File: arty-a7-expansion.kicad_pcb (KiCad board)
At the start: 4 copper layers, 109.4 x 40 mm, 62 parts, among them IC1 TPD8S009DSMR, J2 1140084168, J4 685119134923, J5 UE27AC54100, U1 TPS61232DRCT, U2 MAX3421EEHJ, Y1 ABM8G-12.000MHZ-18-D2Y-T

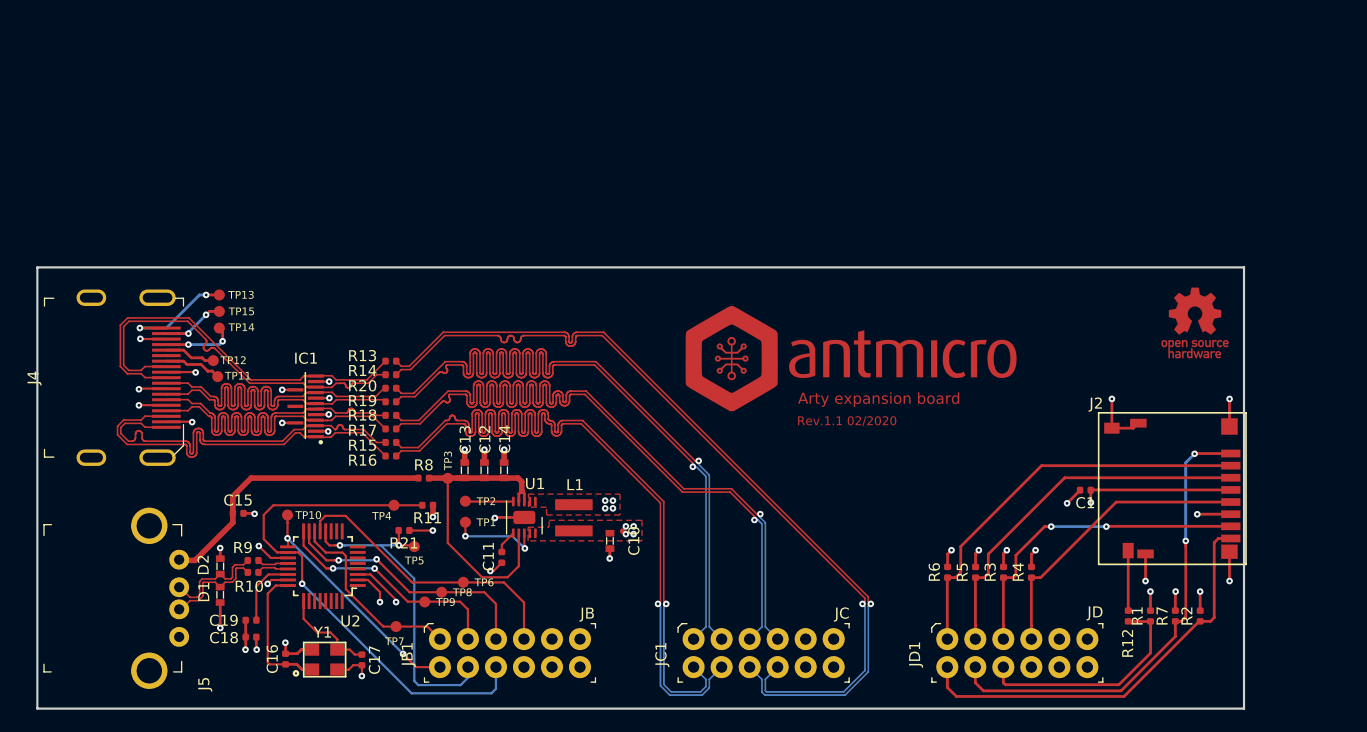
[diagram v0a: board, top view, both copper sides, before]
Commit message: Add revision 2.0.1
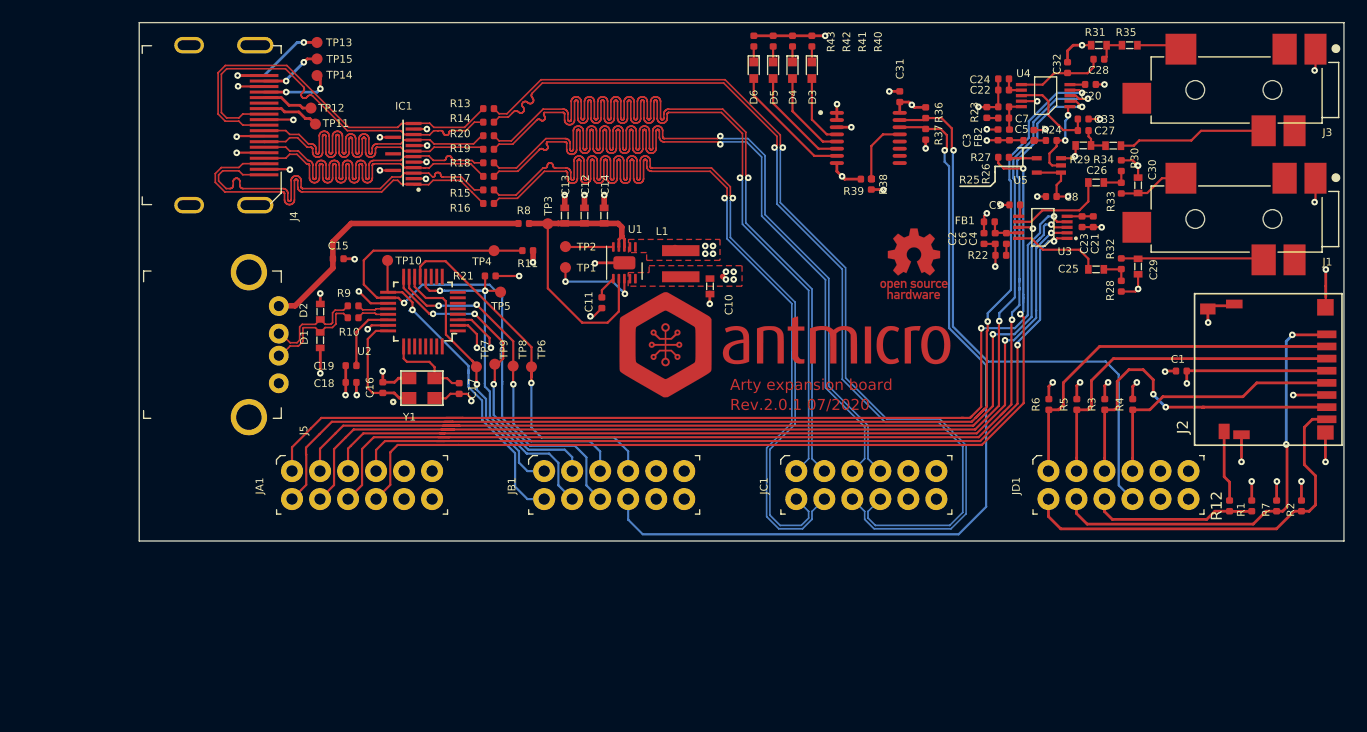
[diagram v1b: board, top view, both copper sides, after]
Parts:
- added C2: C_100n_0402_16V, arty-a7-expansion-footprints:0402-cap, F.Cu at (177.0, 81.9)
- added C20: C_10u_0402, arty-a7-expansion-footprints:0402-cap, F.Cu at (186.6, 67.9)
- added C21: C_100n_0402_16V, arty-a7-expansion-footprints:0402-cap, F.Cu at (186.9, 80.3)
- added C22: C_100n_0402_16V, arty-a7-expansion-footprints:0402-cap, F.Cu at (178.8, 68.4)
- added C23: C_10u_0402, arty-a7-expansion-footprints:0402-cap, F.Cu at (185.9, 80.3)
- added C24: C_1u_0402, arty-a7-expansion-footprints:0402-cap, F.Cu at (178.8, 67.4)
- added C25: C_3u3_0603, arty-a7-expansion-footprints:0603-cap, F.Cu at (187.1, 84.7)
- added C26: C_3u3_0603, arty-a7-expansion-footprints:0603-cap, F.Cu at (187.1, 76.8)
- added C27: C_1u_0402, arty-a7-expansion-footprints:0402-cap, F.Cu at (186.0, 72.1)
- added C28: C_1u_0402, arty-a7-expansion-footprints:0402-cap, F.Cu at (187.4, 65.6)
- added C29: C_2n7_0603, arty-a7-expansion-footprints:0603-cap, F.Cu at (190.9, 84.4)
- added C3: C_100n_0402_16V, arty-a7-expansion-footprints:0402-cap, F.Cu at (178.2, 72.5)
- added C30: C_2n7_0603, arty-a7-expansion-footprints:0603-cap, F.Cu at (190.9, 77.0)
- added C31: C_100n_0402_6V3, arty-a7-expansion-footprints:0402-cap, F.Cu at (169.3, 69.0)
- added C32: C_180p_0402, arty-a7-expansion-footprints:0402-cap, F.Cu at (184.6, 66.4)
- added C33: C_180p_0402, arty-a7-expansion-footprints:0402-cap, F.Cu at (186.0, 71.0)
- added C4: C_4u7_0402, arty-a7-expansion-footprints:0402-cap, F.Cu at (179.0, 81.9)
- added C5: C_4u7_0402, arty-a7-expansion-footprints:0402-cap, F.Cu at (178.8, 70.9)
- added C6: C_100n_0402_16V, arty-a7-expansion-footprints:0402-cap, F.Cu at (178.0, 81.9)
- added C7: C_100n_0402_16V, arty-a7-expansion-footprints:0402-cap, F.Cu at (178.8, 69.9)
- added C8: C_100n_0402_16V, arty-a7-expansion-footprints:0402-cap, F.Cu at (183.1, 78.1)
- added C9: C_10u_0402, arty-a7-expansion-footprints:0402-cap, F.Cu at (179.8, 78.8)
- added D3: LG_L29K-G2J1-24-Z, arty-a7-expansion-footprints:LED_0603, F.Cu at (161.4, 66.6)
- added D4: LG_L29K-G2J1-24-Z, arty-a7-expansion-footprints:LED_0603, F.Cu at (159.6, 66.6)
- added D5: LG_L29K-G2J1-24-Z, arty-a7-expansion-footprints:LED_0603, F.Cu at (157.9, 66.6)
- added D6: LG_L29K-G2J1-24-Z, arty-a7-expansion-footprints:LED_0603, F.Cu at (156.1, 66.6)
- added FB1: BLM15AG601SN1D, arty-a7-expansion-footprints:0402-res, F.Cu at (177.5, 80.3)
- added FB2: BLM15AG601SN1D, arty-a7-expansion-footprints:0402-res, F.Cu at (179.3, 72.5)
- added IC2: PCA9500PW, arty-a7-expansion-footprints:TSSOP-16, F.Cu at (166.5, 72.7)
- added J1: SJ-43516-SMT-GR, arty-a7-expansion-footprints:CUI_SJ-43516-SMT-GR, F.Cu at (199.9, 80.1)
- added J3: SJ-43516-SMT-BE, arty-a7-expansion-footprints:CUI_SJ-43516-SMT-BE, F.Cu at (199.9, 68.4)
- added JA1: 10883121, arty-a7-expansion-footprints:PinHeader_6x2_P2.54mm_Horizontal_Mirrored, F.Cu at (114.2, 102.7)
- added R22: R_1R_0402, arty-a7-expansion-footprints:0402-res, F.Cu at (178.5, 83.4)
- added R23: R_1R_0402, arty-a7-expansion-footprints:0402-res, F.Cu at (177.2, 70.4)
- added R24: R_10k_0402, arty-a7-expansion-footprints:0402-res, F.Cu at (183.1, 73.0)
- added R25: R_0R_0402, arty-a7-expansion-footprints:0402-res, F.Cu at (181.0, 73.0)
- added R26: R_0R_0402, arty-a7-expansion-footprints:0402-res, F.Cu at (181.5, 72.5)
- added R27: R_0R_0402, arty-a7-expansion-footprints:0402-res, F.Cu at (178.8, 74.5)
- added R28: R_10k_0402, arty-a7-expansion-footprints:0402-res, F.Cu at (189.4, 86.2)
- added R29: R_5k1_0603, arty-a7-expansion-footprints:0603-res, F.Cu at (186.0, 73.4)
- added R30: R_10k_0402, arty-a7-expansion-footprints:0402-res, F.Cu at (189.4, 75.3)
- added R31: R_5k1_0603, arty-a7-expansion-footprints:0603-res, F.Cu at (187.4, 64.3)
- added R32: R_470R_0402, arty-a7-expansion-footprints:0402-res, F.Cu at (189.4, 84.1)
- added R33: R_470R_0402, arty-a7-expansion-footprints:0402-res, F.Cu at (189.4, 77.3)
- added R34: R_5k1_0603, arty-a7-expansion-footprints:0603-res, F.Cu at (188.7, 73.4)
- added R35: R_5k1_0603, arty-a7-expansion-footprints:0603-res, F.Cu at (190.2, 64.3)
- added R36: R_2k_0402, arty-a7-expansion-footprints:0402-res, F.Cu at (171.7, 70.5)
- added R37: R_2k_0402, arty-a7-expansion-footprints:0402-res, F.Cu at (171.7, 72.4)
- added R38: R_100k_0402, arty-a7-expansion-footprints:0402-res, F.Cu at (166.8, 76.9)
- added R39: R_0R_0402, arty-a7-expansion-footprints:0402-res, F.Cu at (166.3, 76.5)
- added R40: R_100R_0402, arty-a7-expansion-footprints:0402-res, F.Cu at (161.4, 64.0)
- added R41: R_100R_0402, arty-a7-expansion-footprints:0402-res, F.Cu at (159.6, 64.0)
- added R42: R_100R_0402, arty-a7-expansion-footprints:0402-res, F.Cu at (157.9, 64.0)
- added R43: R_100R_0402, arty-a7-expansion-footprints:0402-res, F.Cu at (156.1, 64.0)
- added U3: CS4344-CZZ, arty-a7-expansion-footprints:10TSSOP, F.Cu at (182.3, 80.8)
- added U4: CS5343-CZZ, arty-a7-expansion-footprints:10TSSOP, F.Cu at (182.6, 68.9)
- added U5: NC7SZ126P5X, arty-a7-expansion-footprints:SC-70-5, F.Cu at (182.9, 75.2)
- JB1, JC1, JD1: value 0015912120 -> 10883121
- L1: value XFL4020-102MEB -> XFL4020-102MEC
- moved C16 26.1 mm to (122.5, 95.4)
- moved Y1 26.1 mm to (126.0, 95.4)
- moved C17 26.1 mm to (129.4, 95.5)
- moved N2 26.0 mm to (170.6, 84.1)
- moved L1 25.0 mm to (149.5, 84.1), turned to 90 degrees
- moved C10 24.8 mm to (152.1, 86.2)
- moved D1 24.8 mm to (116.8, 91.1)
- moved R11 24.8 mm to (135.6, 83.0)
- moved C11 24.8 mm to (142.3, 87.7)
- moved C14 24.8 mm to (142.5, 79.8)
- moved C15 24.8 mm to (118.4, 83.7)
- moved C19 24.8 mm to (119.6, 94.9)
- moved D2 24.8 mm to (116.8, 88.5)
- moved TP1 24.8 mm to (139.0, 84.4)
- moved TP10 24.8 mm to (122.9, 83.8)
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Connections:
- JB1 pad 10: Net-(JB1-Pad10) -> /GPIO_SCL
- JD1 pad 10: /NC_EN -> /GPIO_SDA
- L1 pad 1: Net-(L1-Pad1) -> +3V3
- L1 pad 2: +3V3 -> Net-(L1-Pad2)
- U1 pad 1: Net-(L1-Pad1) -> Net-(L1-Pad2)
- U1 pad 2: Net-(L1-Pad1) -> Net-(L1-Pad2)
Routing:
- net /ADIN_MCLK: track 0.00 -> 105.2 mm, vias 0 -> 2
- net /ADIN_LRCK: track 0.00 -> 103.0 mm, vias 0 -> 2
- net /ADIN_SCLK: track 0.00 -> 100.3 mm, vias 0 -> 2
- net /ADOUT_MCLK: track 0.00 -> 91.5 mm, vias 0 -> 2
- net /ADIN_SDOUT: track 0.00 -> 89.3 mm, vias 0 -> 2
- net /ADOUT_LRCK: track 0.00 -> 88.3 mm, vias 0 -> 2
- net /ADOUT_SCLK: track 0.00 -> 82.7 mm, vias 0 -> 2
- net /ADOUT_SDIN: track 0.00 -> 80.0 mm, vias 0 -> 2
- net /GPIO_SCL: track 0.00 -> 76.0 mm, vias 0 -> 1
- net /GPIO_SDA: track 0.00 -> 52.0 mm, vias 0 -> 1
- net GND: track 65.1 -> 104.3 mm, vias 29 -> 49
- net +3V3: track 38.5 -> 62.6 mm, vias 19 -> 27
- net Net-(J3-Pad3): track 0.00 -> 13.5 mm
- net Net-(C29-Pad1): track 0.00 -> 13.0 mm
- net Net-(D6-Pad2): track 0.00 -> 11.3 mm
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- added copper zone on F.Cu, net Net-(L1-Pad2)
- removed copper zone on F.Cu, net Net-(L1-Pad1)
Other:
- board size 109.4 x 40 mm -> 109.2 x 47 mm
- board text added: "Rev.2.0.1 07/2020"
- board text removed: "JB"
- board text removed: "JC"
- board text removed: "JD"
- board text removed: "Rev.1.1 02/2020"
